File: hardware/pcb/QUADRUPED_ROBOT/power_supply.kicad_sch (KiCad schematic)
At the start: 54 parts, among them J10 PIN, J3 SWITCH_POWER, J5 PIN, J7 USB_A, J9 JETSON, Q1 AO4485, U1 XL4016, U3 TPS5430DDA

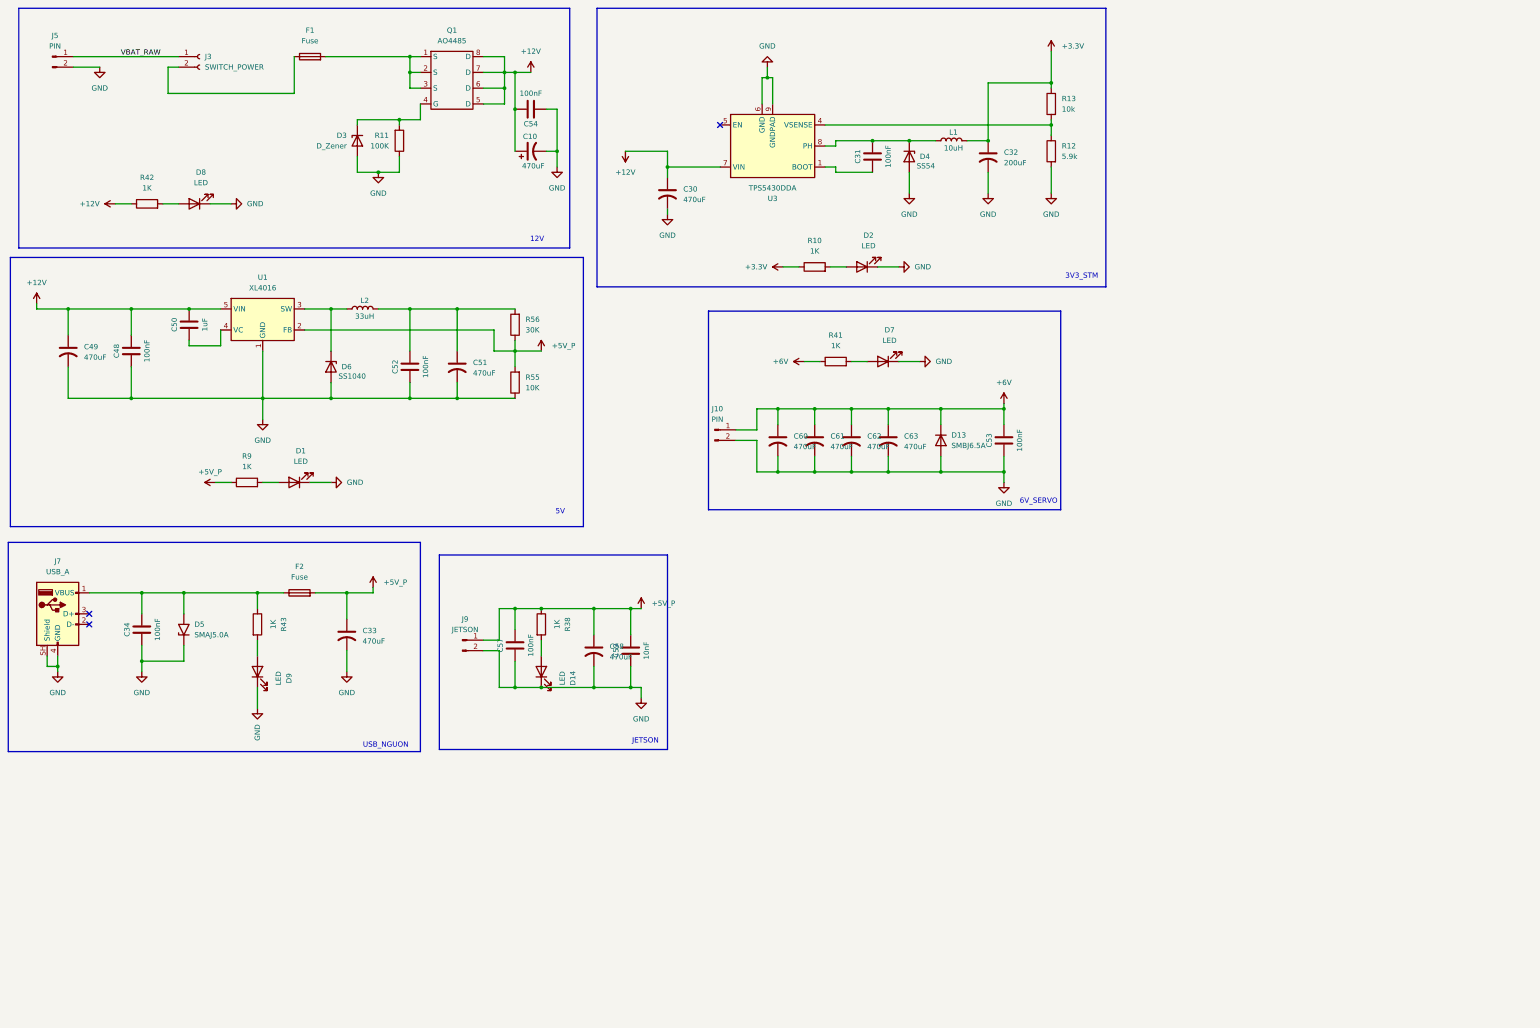
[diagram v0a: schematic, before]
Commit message: pcb update
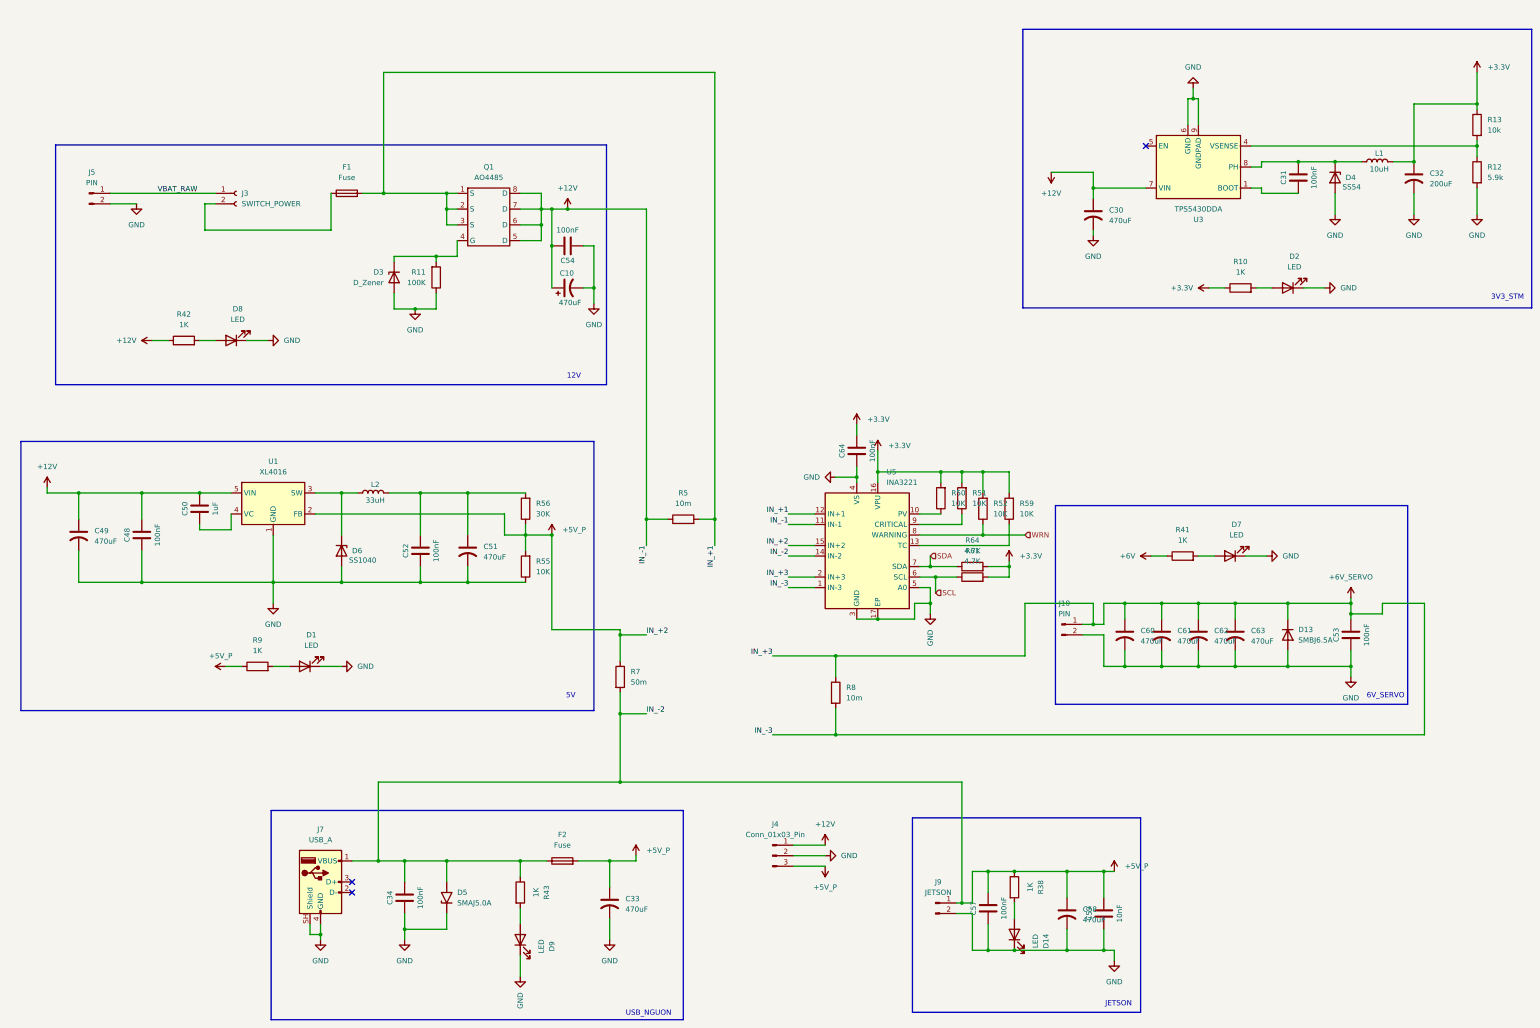
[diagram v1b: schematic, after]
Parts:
- added C64: 100nF, Capacitor_SMD:C_0805_2012Metric, symbol Device:C
- added J4: Conn_01x03_Pin, Connector_PinHeader_2.54mm:PinHeader_1x03_P2.54mm_Vertical, symbol Connector:Conn_01x03_Pin
- added R5, R8: 10m, Resistor_SMD:R_2512_6332Metric, symbol Device:R
- added R50, R51, R52, R59: 10K, Resistor_SMD:R_0805_2012Metric, symbol Device:R
- added R61, R64: 4.7K, Resistor_SMD:R_0805_2012Metric, symbol Device:R
- added R7: 50m, Resistor_SMD:R_2512_6332Metric, symbol Device:R
- added U5: INA3221, Package_DFN_QFN:Texas_RGV0016A_VQFN-16-1EP_4x4mm_P0.65mm_EP2.1x2.1mm, symbol Power_Management:INA3221
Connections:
- net +12V: now also J4.1 (Pin_1), R5.1, U5.11 (IN-1)
- net +3.3V: now also C64.2, R50.2, R51.2, R52.2, R59.2, R61.2, R64.2, U5.16 (VPU)
- net +5V_P: now also C34.2, D5.2 (A2), F2.1, J7.1 (VBUS), R43.1, J4.3 (Pin_3), R7.1, R7.2, U5.14 (IN-2), U5.15 (IN+2)
- net +6V: no longer C53.2, C60.1, C61.1, C62.1, C63.1, D13.1 (K), J10.1 (Pin_1)
- net GND: now also C64.1, J4.2 (Pin_2), U5.17 (EP), U5.3 (GND), U5.4 (VS), U5.5 (A0)
- net IN_+1: now reaches F1.2, Q1.1 (S), Q1.2 (S), Q1.3 (S)
- net IN_+1: now also R5.2, U5.12 (IN+1)
- new net: R59.1, U5.13 (TC)
- new net: R50.1, U5.10 (PV)
- new net: R51.1, U5.9 (CRITICAL)
- new net +6V_SERVO: C53.2, C60.1, C61.1, C62.1, C63.1, D13.1 (K), J10.1 (Pin_1), R8.1, R8.2, U5.1 (IN-3), U5.2 (IN+3)
- new net SCL: R61.1, U5.6 (SCL)
- new net SDA: R64.1, U5.7 (SDA)
- new net WRN: R52.1, U5.8 (WARNING)
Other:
- moved on the sheet: C10, C30, C31, C32, C33, C34, C48, C49, C50, C51, C52, C53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
